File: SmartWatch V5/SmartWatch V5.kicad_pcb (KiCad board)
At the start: 4 copper layers, 31.9 x 34.2 mm, 60 parts, among them J1 10118192-0001LF, J10 TestPad, J2 , J7 TestPad, J8 TestPad, J9 TestPad, Q1 FDN340P, Q2 MMBT3904, Q3 MMBT3904, Q4 FDN028N20, Q5 FDN028N20, Q6 FDN028N20, SW1 EVQ-P7J01P, SW2 EVQ-P7J01P, U1 MAX17260, U10 TSC2003IPWR, U2 FT231XQ, U3 LP5912-3.3DRVT, U5 MCP73832-2-OT, U6 ESP32-WROOM-32, U8 ADXL337

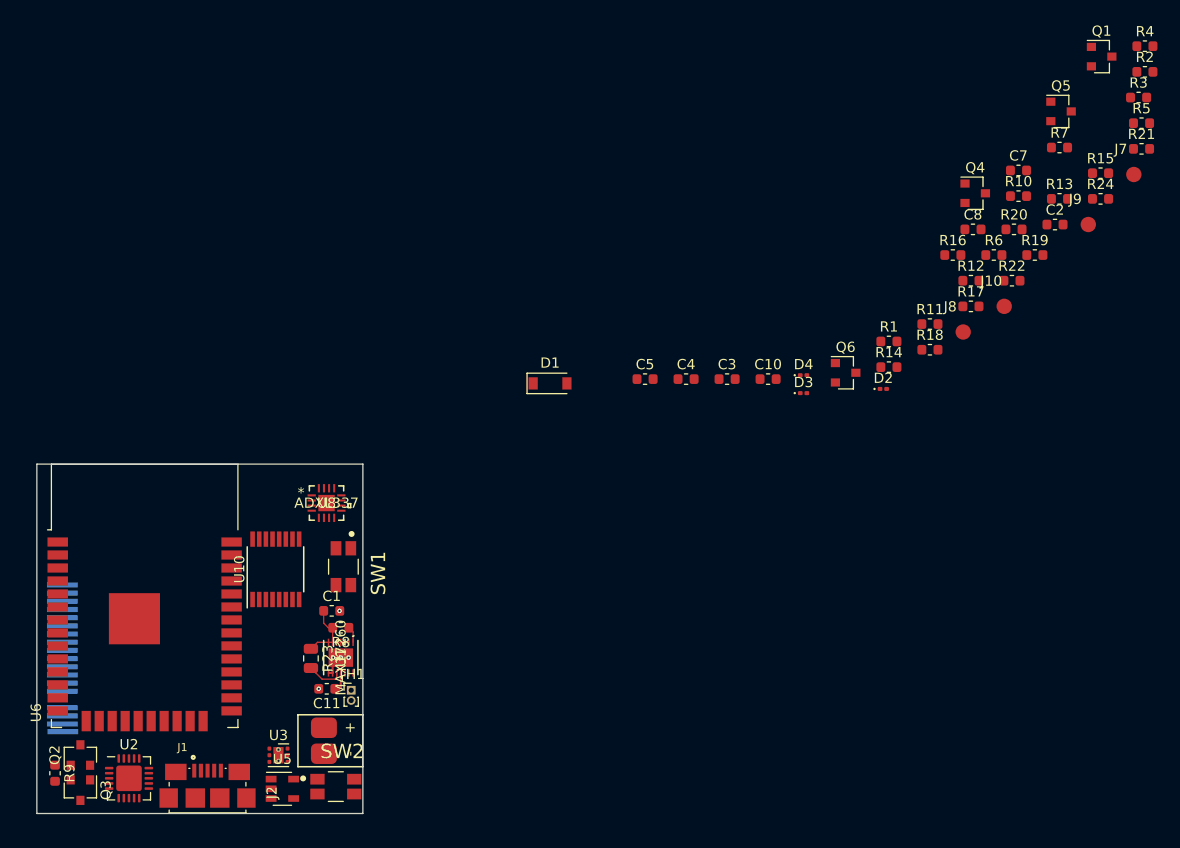
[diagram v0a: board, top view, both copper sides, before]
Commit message: Layout Work on Rev 5
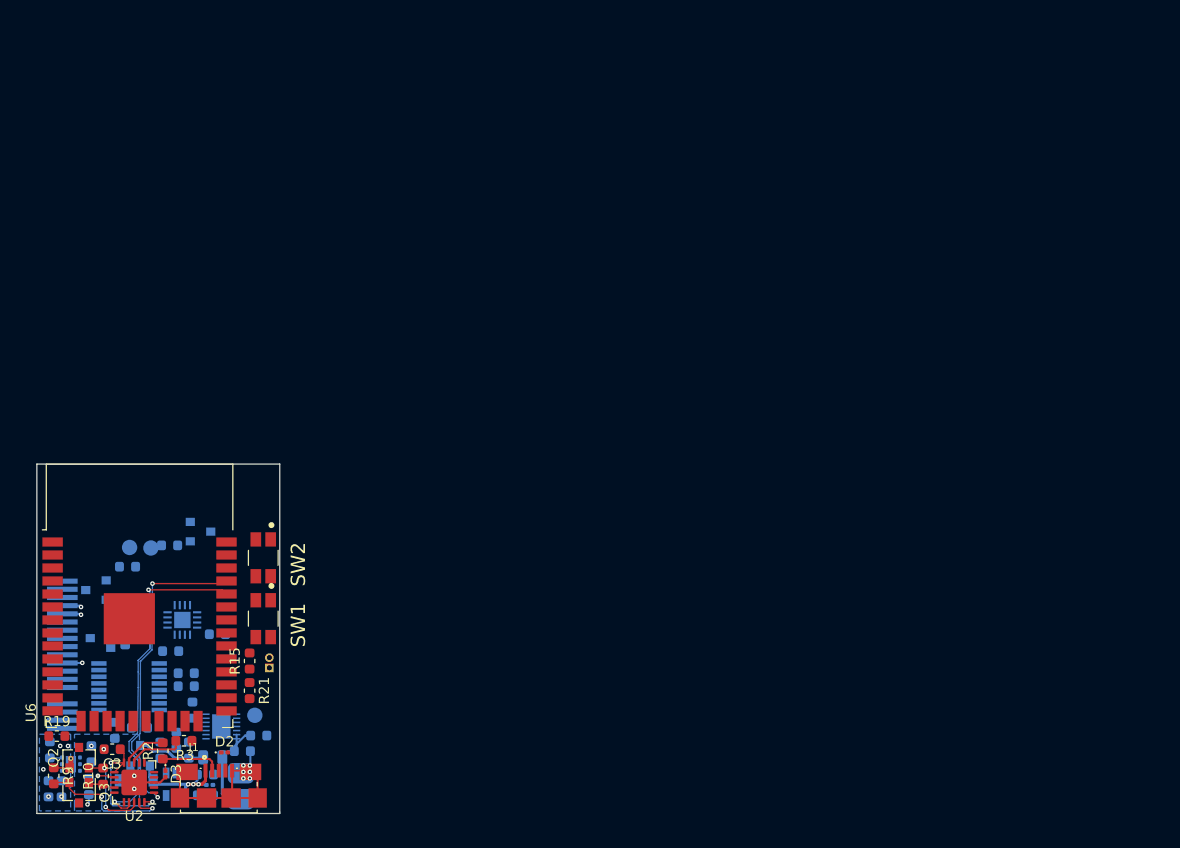
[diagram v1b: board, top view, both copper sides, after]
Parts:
- removed J7: TestPad, CustomFootprints:TESTPAD
- removed R11, R12: 0, Resistor_SMD:R_0603_1608Metric
- C1, C10, C11, C2, C4, C5, C7, C8, D1, D4, J10, J2, J8, J9, Q1, Q4, Q5, Q6, R1, R13, R14, R16, R17, R18, R20, R22, R23, R24, R4, R5, R6, R7, R8, TH1, U1, U10, U3, U5, U8: moved to B.Cu
- moved R4 120.9 mm to (88.5, 91.7), turned to 90 degrees
- moved R2 116.7 mm to (93.2, 93.7), turned to 90 degrees
- moved Q1 116.2 mm to (91.0, 94.2), turned to 90 degrees
- moved R7 114.9 mm to (82.2, 93.6), turned to 270 degrees
- moved R5 114.4 mm to (90.9, 91.4)
- moved R3 112.5 mm to (95.3, 92.7), turned to 180 degrees
- moved C2 109.3 mm to (86.0, 97.2), turned to 270 degrees
- moved R19 106.6 mm to (82.9, 92.3)
- moved R10 105.9 mm to (87.4, 96.2), turned to 90 degrees
- moved C8 105.6 mm to (82.0, 97.4), turned to 270 degrees
- moved Q5 105.3 mm to (86.7, 78.0), turned to 180 degrees
- moved R21 102.0 mm to (101.7, 87.8), turned to 270 degrees
- moved R24 101.7 mm to (89.8, 75.7)
- moved C7 99.0 mm to (95.8, 93.6), turned to 90 degrees
- moved R13 97.2 mm to (95.5, 86.1), turned to 180 degrees
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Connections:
- U2 pad 17: /TXD -> /RXD0
- U6 pad 28: (no net) -> /ACCEL_EN
- U6 pad 35: /TXD0 -> /RXD
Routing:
- net /RXD0: track 0.00 -> 35.2 mm, vias 0 -> 2
- net /RXD: track 0.00 -> 31.3 mm, vias 0 -> 2
- net GND: track 2.23 -> 27.5 mm, vias 5 -> 13
- net /RTS: track 0.00 -> 13.8 mm, vias 0 -> 2
- net Net-(C3-Pad1): track 0.00 -> 13.2 mm, vias 0 -> 2
- net /VBUS: track 0.00 -> 12.1 mm, vias 0 -> 3
- net /DTR: track 0.00 -> 8.88 mm, vias 0 -> 2
- net +3V3: track 0.00 -> 7.38 mm, vias 0 -> 7
- net Net-(D3-Pad1): track 0.00 -> 7.06 mm
- net Net-(R3-Pad2): track 0.00 -> 5.30 mm
- net /BAT+: track 6.09 -> 11.2 mm
- net Net-(R2-Pad2): track 0.00 -> 4.35 mm
- net /BAT_SENSE: track 3.49 -> 6.71 mm
- net /MAX_REG: track 2.17 -> 0.00 mm
- net Net-(R8-Pad1): track 1.59 -> 0.00 mm
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- added copper zone on B.Cu, net +3V3
- added copper zone on In2.Cu, net +3V3
- added copper zone on B.Cu, net /PWR_IN
- added copper zone on In1.Cu, net GND
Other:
- board size 31.9 x 34.2 mm -> 23.7 x 34.2 mm
- net class Default: clearance 0.2 -> 0.1; trace_width 0.25 -> 0.1; via_dia 0.8 -> 0.45; via_drill 0.4 -> 0.2
- rule trace_clearance: 0.2 -> 0.1
